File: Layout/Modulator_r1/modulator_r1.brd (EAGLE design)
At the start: 68.2 x 40.6 mm, 21 parts, among them IC1 FT232RL, U1 ATMEGA328P-AU, U2 TPS79933QDDCRQ1

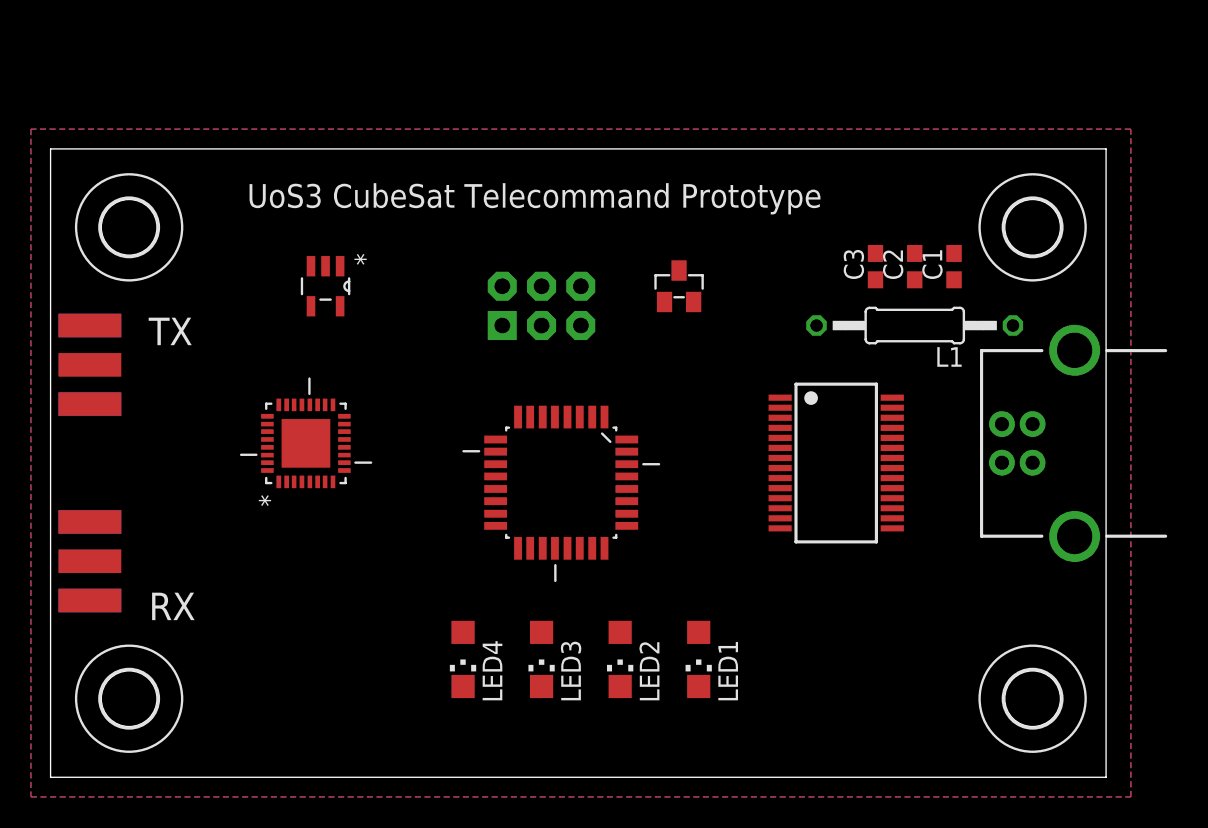
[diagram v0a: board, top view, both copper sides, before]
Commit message: Layout progress.
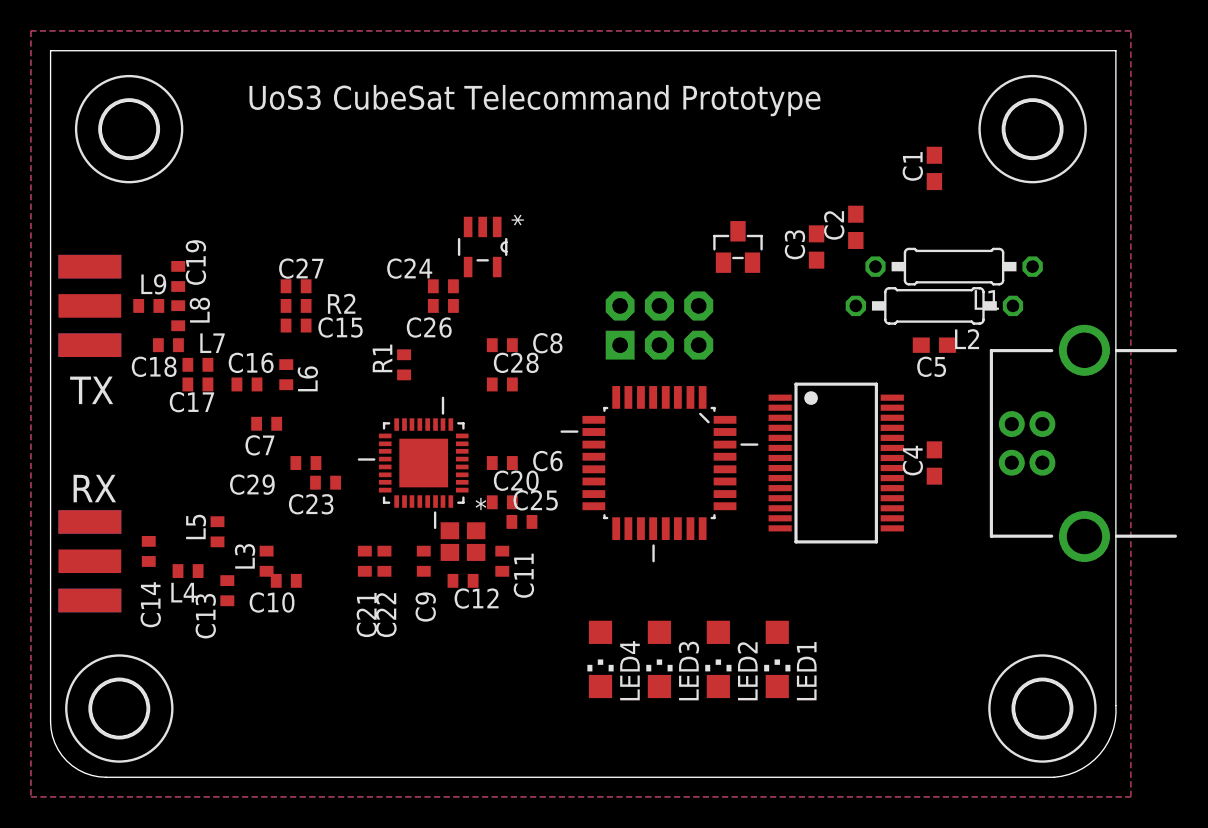
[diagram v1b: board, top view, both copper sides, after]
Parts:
- added C10: 1n8, resistor:C0402
- added C11, C12: 12p, resistor:C0402
- added C13, C14, C18: 5p1, resistor:C0402
- added C15: 56p, resistor:C0402
- added C16: 39p, resistor:C0402
- added C17: 2p2, resistor:C0402
- added C19: 6p2, resistor:C0402
- added C20, C21, C22, C23, C24, C25, C26, C28, C29, C8, C9: 47n, resistor:C0402
- added C27: 100p, resistor:C0402
- added C4: 100nF, resistor:C0603
- added C5: 10nF, resistor:C0603
- added C6: 220n, resistor:C0402
- added C7: 10n, resistor:C0402
- added L2: FB, resistor:0207/10
- added L3, L6: 56n, resistor:R0402
- added L4, L5: 27n, resistor:R0402
- added L7: 15n, resistor:R0402
- added L8: 43n, resistor:R0402
- added L9: 22n, resistor:R0402
- added Q1: FA-20H, crystal:FA-20H
- added R1: 56K, resistor:R0402
- added R2: 18R, resistor:R0402
- L1: device resistor:0207/12 -> resistor:0207/10
- moved J$2 16.5 mm to (2.54, 27.9)
- moved J$1 12.7 mm to (2.54, 11.4)
- moved U2 10.5 mm to (27.9, 34.3)
- moved LED4 8.89 mm to (35.6, 7.62)
- moved JP1 7.73 mm to (39.4, 29.2)
- moved U$1 7.73 mm to (24.1, 20.3), turned to 180 degrees
- moved LED3 7.62 mm to (39.4, 7.62)
- moved C1 6.48 mm to (57.1, 39.4)
- moved U1 6.48 mm to (39.4, 20.3)
- moved LED2 6.35 mm to (43.2, 7.62)
- moved U$4 6.35 mm to (63.5, 41.9)
- moved U$5 6.35 mm to (5.08, 41.9)
- moved LED1 5.08 mm to (47.0, 7.62)
- moved C2 4.58 mm to (52.1, 35.6)
- moved L1 4.58 mm to (58.4, 33.0)
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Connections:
- new net CC_IO0: U$1.10
- new net CC_IO2: U$1.4
- new net CC_IO3: U$1.3
- new net CC_LNA_N: C13.2, L3.1, L4.1, U$1.20
- new net CC_LNA_P: C14.1, L3.2, L5.1, U$1.19
- new net CC_NRESET: U$1.2
- new net CC_RF_PA: C16.2, L6.2, U$1.17
- new net CC_VDD: C15.1, C20.1, C21.1, C22.1, C23.1, C24.1, C25.1, C26.1, C27.1, C28.1, C29.1, R2.2, U$1.1, U$1.12, U$1.13, U$1.15, U$1.22, U$1.25, U$1.27, U$1.28, U$1.5, U2.5
- new net N$10: C7.1, U$1.21
- new net N$11: C6.1, U$1.6
- new net N$12: C10.2, U$1.24
- new net N$13: C10.1, U$1.23
- new net N$14: C11.1, Q1.1, U$1.31
- new net N$15: C19.1, L8.1, L9.2
- new net N$16: C12.1, Q1.3, U$1.30
- new net N$17: C14.2, J$1.SIG, L4.2
- new net N$18: C17.1, C18.1, L7.1, L8.2
- new net N$19: C16.1, C17.2, L7.2
- new net N$21: C15.2, L6.1, R2.1
- new net N$4: C5.1, JP2.VBUS, L2.1
- new net N$5: C4.1, IC1.17
- new net N$6: J$2.SIG, L9.1
- new net N$7: R1.1, U$1.14
- new net N$8: C9.1, U$1.29
- new net N$9: C8.1, U$1.26
- net GND: now also C11.2, C12.2, C13.1, C18.2, C19.2, C20.2, C21.2, C22.2, C23.2, C24.2, C25.2, C26.2, C27.2, C28.2, C29.2, C4.2, C5.2, C6.2, C7.2, C8.2, C9.2, IC1.26, L5.2, Q1.2, Q1.4, R1.2
- net VCCIO: now also L2.2; no longer JP2.VBUS
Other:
- board size 68.2 x 40.6 mm -> 68.9 x 47 mm
